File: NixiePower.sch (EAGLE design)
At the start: 14 parts, among them IC1 MC34063AD

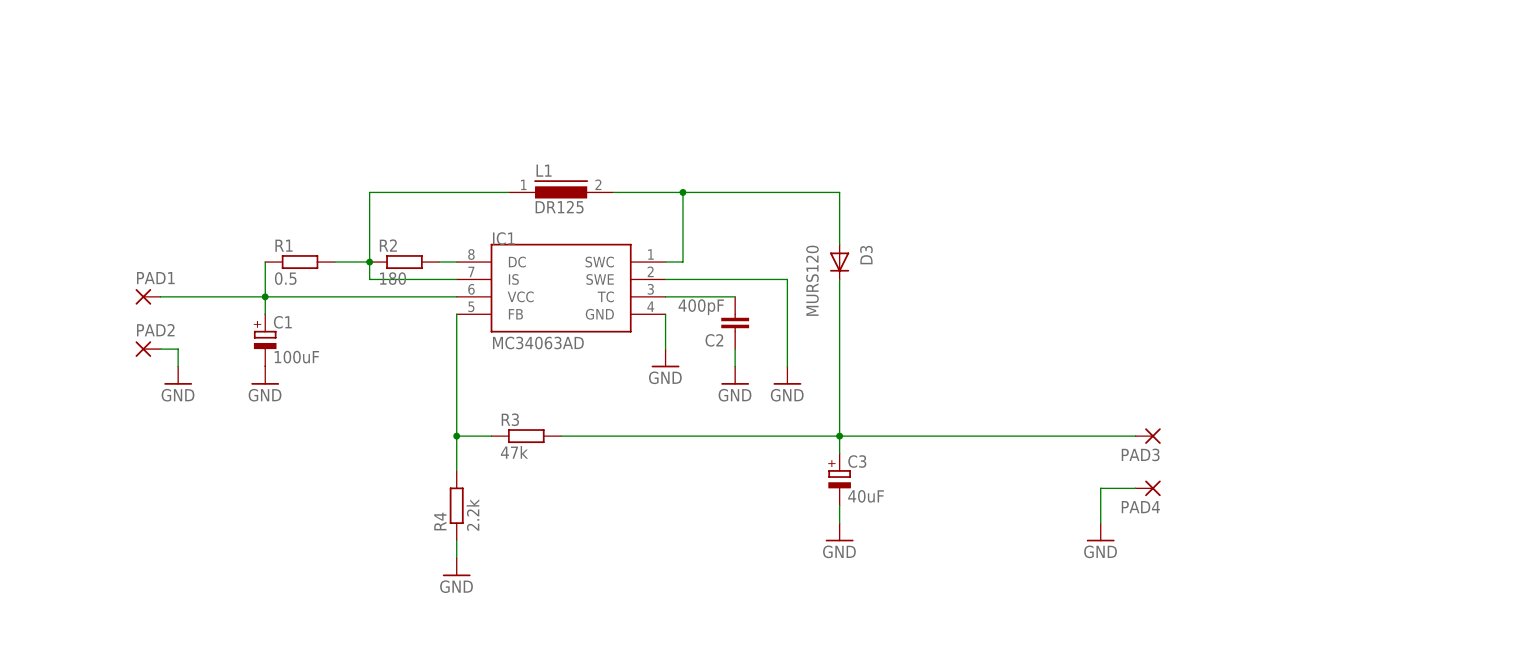
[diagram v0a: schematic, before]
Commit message: Commit of Rev.B version
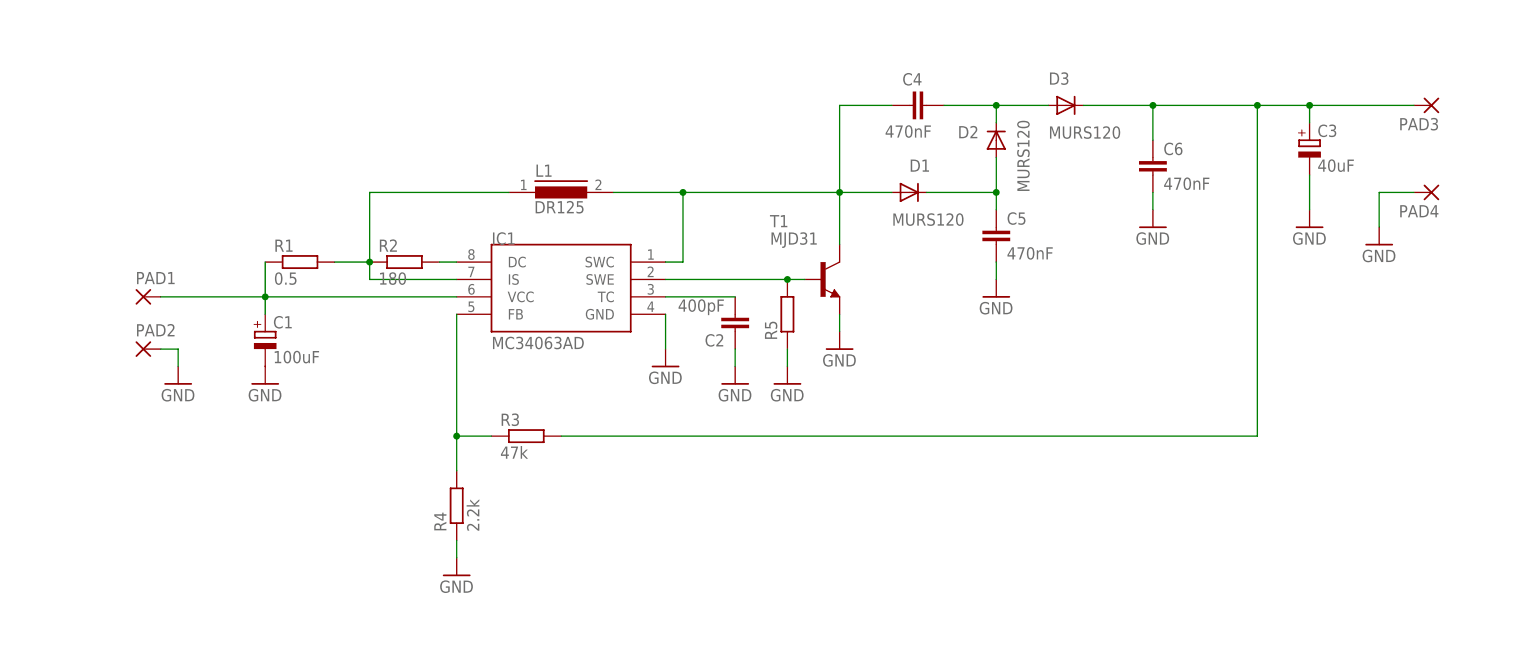
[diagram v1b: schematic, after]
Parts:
- added C4, C5, C6: 470nF, rcl:C-EUC1206K
- added D1, D2: MURS120, diode:DIODE-DO214AA
- added R5: (no value), rcl-2:R-EU_R1206
- added T1: MJD31, transistor:MJD31
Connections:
- removed net N$6: C3.+, D3.C, PAD3.P, R3.2
- new net N$10: C3.+, C6.1, D3.C, PAD3.P, R3.2
- new net N$11: IC1.SWE, R5.2, T1.B
- new net N$8: C5.1, D1.C, D2.A
- new net N$9: C4.1, D2.C, D3.A
- net GND: now also C5.2, C6.2, R5.1, T1.E; no longer IC1.SWE
- net N$1: now also C4.2, D1.A, T1.C; no longer D3.A
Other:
- moved on the sheet: C3, D3, PAD3, PAD4

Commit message: Commit of Rev.C version
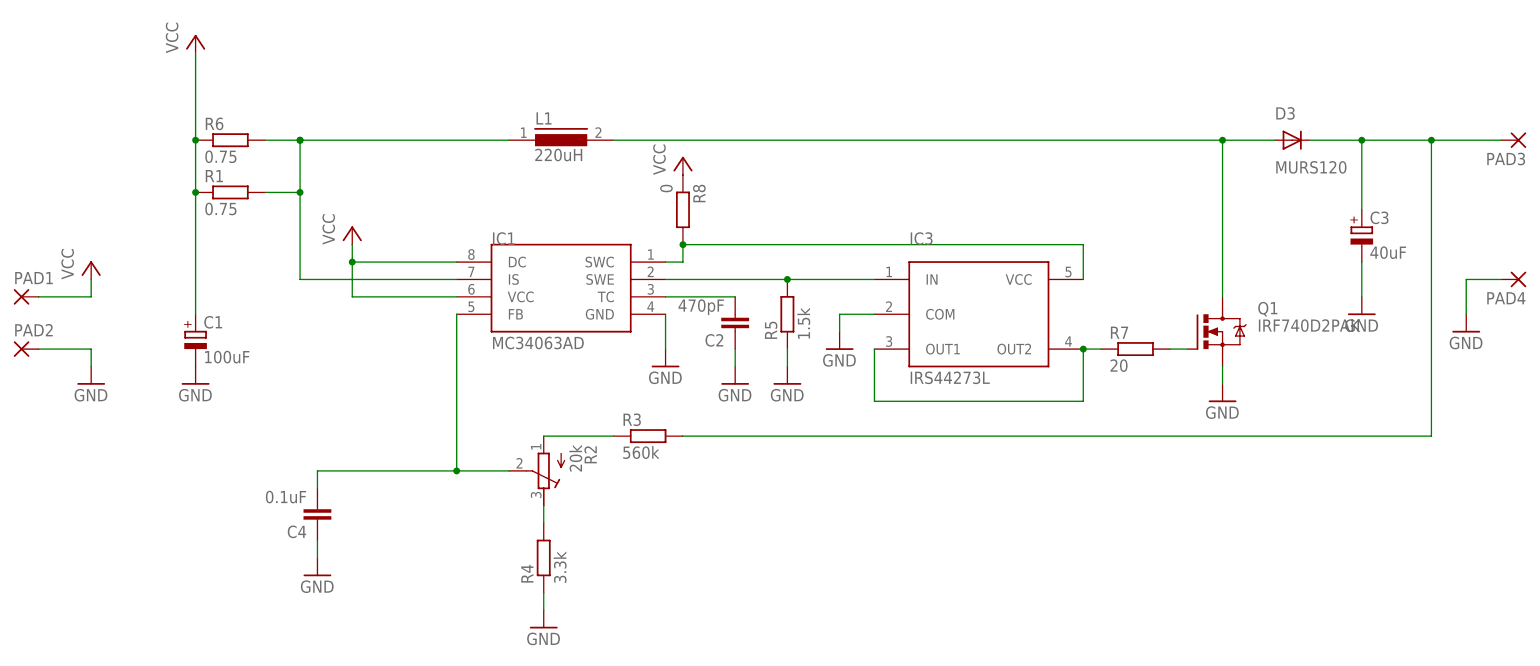
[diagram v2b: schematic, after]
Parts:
- removed C5, C6: 470nF, rcl:C-EUC1206K
- removed D1, D2: MURS120, diode:DIODE-DO214AA
- removed T1: MJD31, transistor:MJD31
- added IC3: IRS44273L, own-collection:IRS44273L
- added Q1: IRF740D2PAK, own-collection:IRF740D2PAK
- added R6: 0.75, rcl-2:R-EU_R1206
- added R7: 20, rcl-2:R-EU_R1206
- added R8: 0, rcl-2:R-EU_R1206
- C2: value 400pF -> 470pF
- C4: value 470nF -> 0.1uF
- L1: value DR125 -> 220uH
- R1: value 0.5 -> 0.75
- R2: value 180 -> 20k; device rcl-2:R-EU_R1206 -> rcl:R-TRIMM4G/J
- R3: value 47k -> 560k
- R4: value 2.2k -> 3.3k
- R5: value (none) -> 1.5k
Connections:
- new net N$6: C3.+, D3.C, PAD3.P, R3.2
- new net VCC: C1.+, IC1.DC, IC1.VCC, PAD1.P, R1.1, R6.1, R8.1
- net GND: now also C4.1, IC3.COM, Q1.S; no longer C5.2, C6.2, T1.E
- net N$1: now also D3.A, Q1.D; no longer C4.2, D1.A, IC1.SWC, T1.C
- net N$10: now also R2.E, R4.2; no longer C3.+, C6.1, D3.C, PAD3.P, R3.2
- net N$11: now also IC3.IN; no longer T1.B
- net N$3: now also R6.2; no longer R2.1
- net N$4: now also IC1.SWC, IC3.VCC, R8.2; no longer IC1.DC, R2.2
- net N$5: now also Q1.G, R7.2; no longer C1.+, IC1.VCC, PAD1.P, R1.1
- net N$7: now also C4.2, R2.S; no longer R3.1, R4.2
- net N$8: now also IC3.OUT1, IC3.OUT2, R7.1; no longer C5.1, D1.C, D2.A
- net N$9: now also R2.A, R3.1; no longer C4.1, D2.C, D3.A
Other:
- moved on the sheet: C1, C3, C4, D3, L1, PAD1, PAD2, PAD3, PAD4, R1, R3, R4
